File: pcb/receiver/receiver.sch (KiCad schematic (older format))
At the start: 30 parts, among them Q101 Q_PMOS_DSG, U101 TPS63700DRCR, U102 NCP1403SNT1G

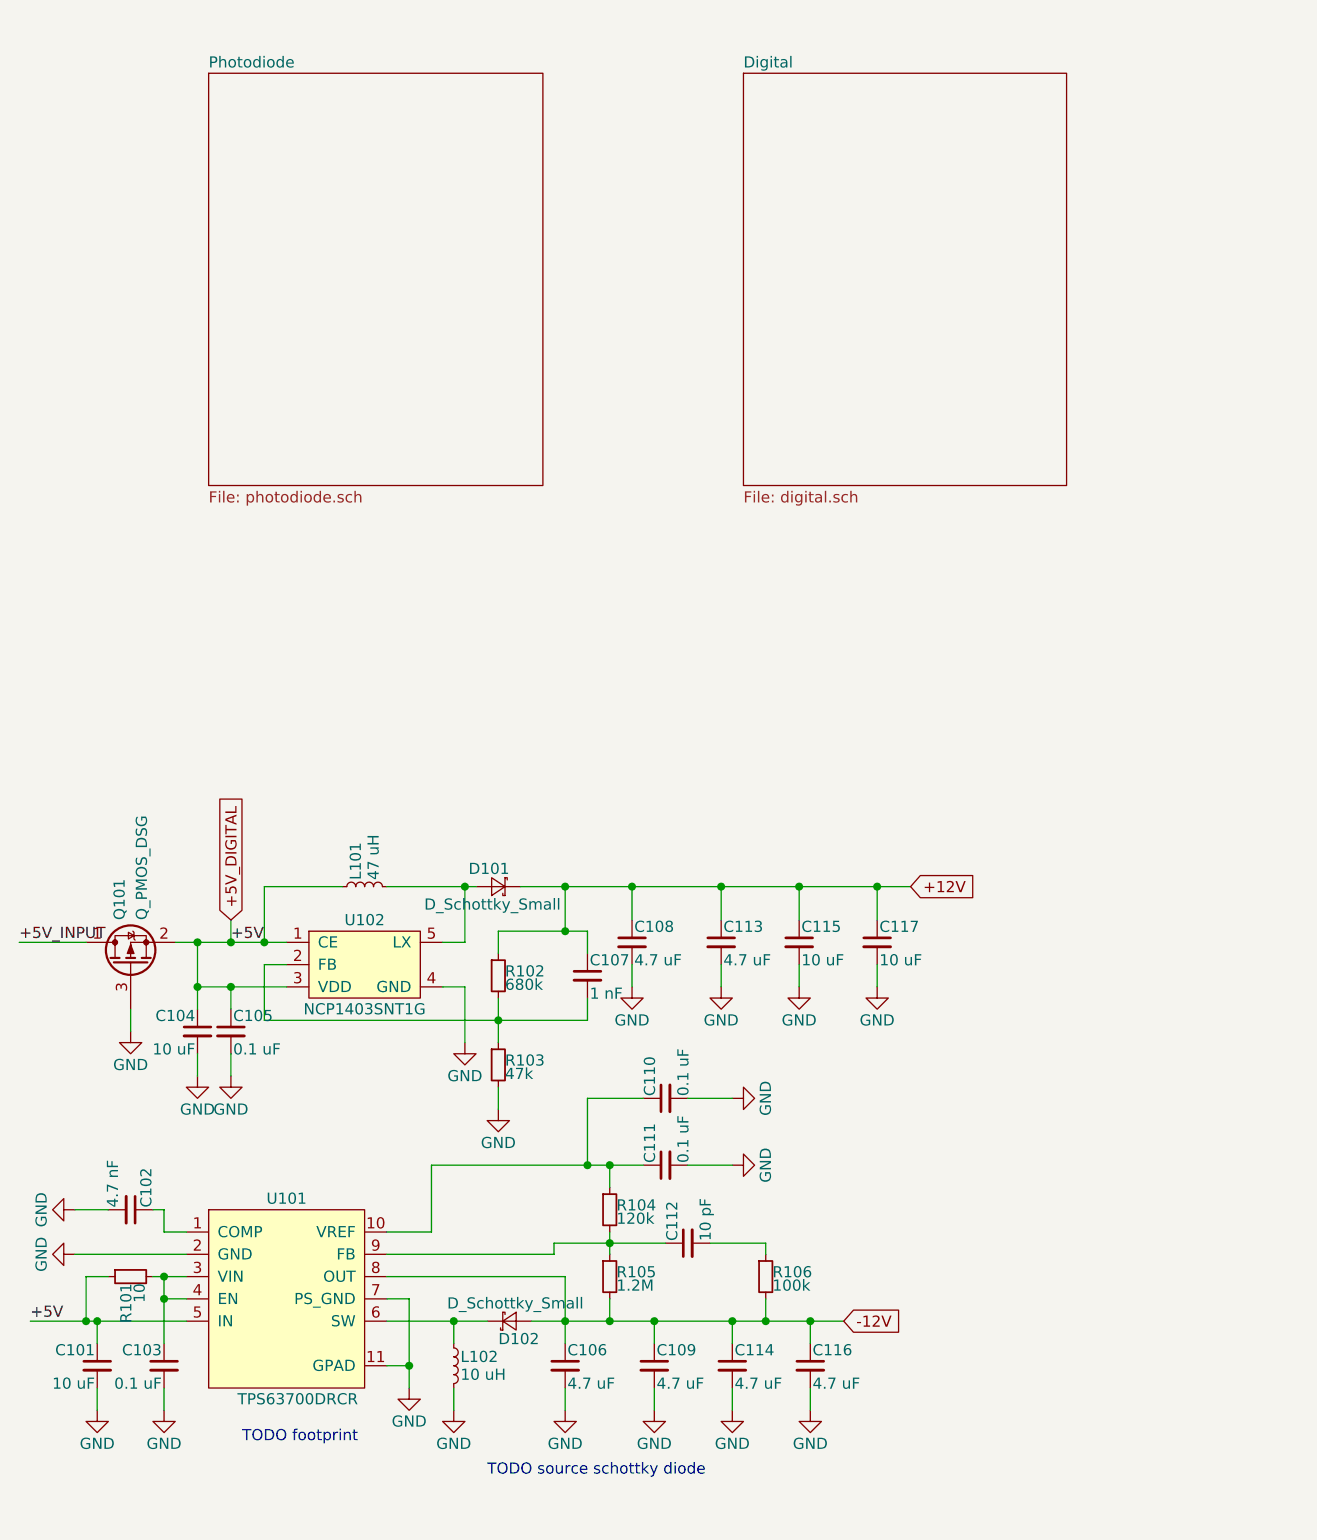
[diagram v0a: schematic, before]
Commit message: Add all components TODO footprint/source everything
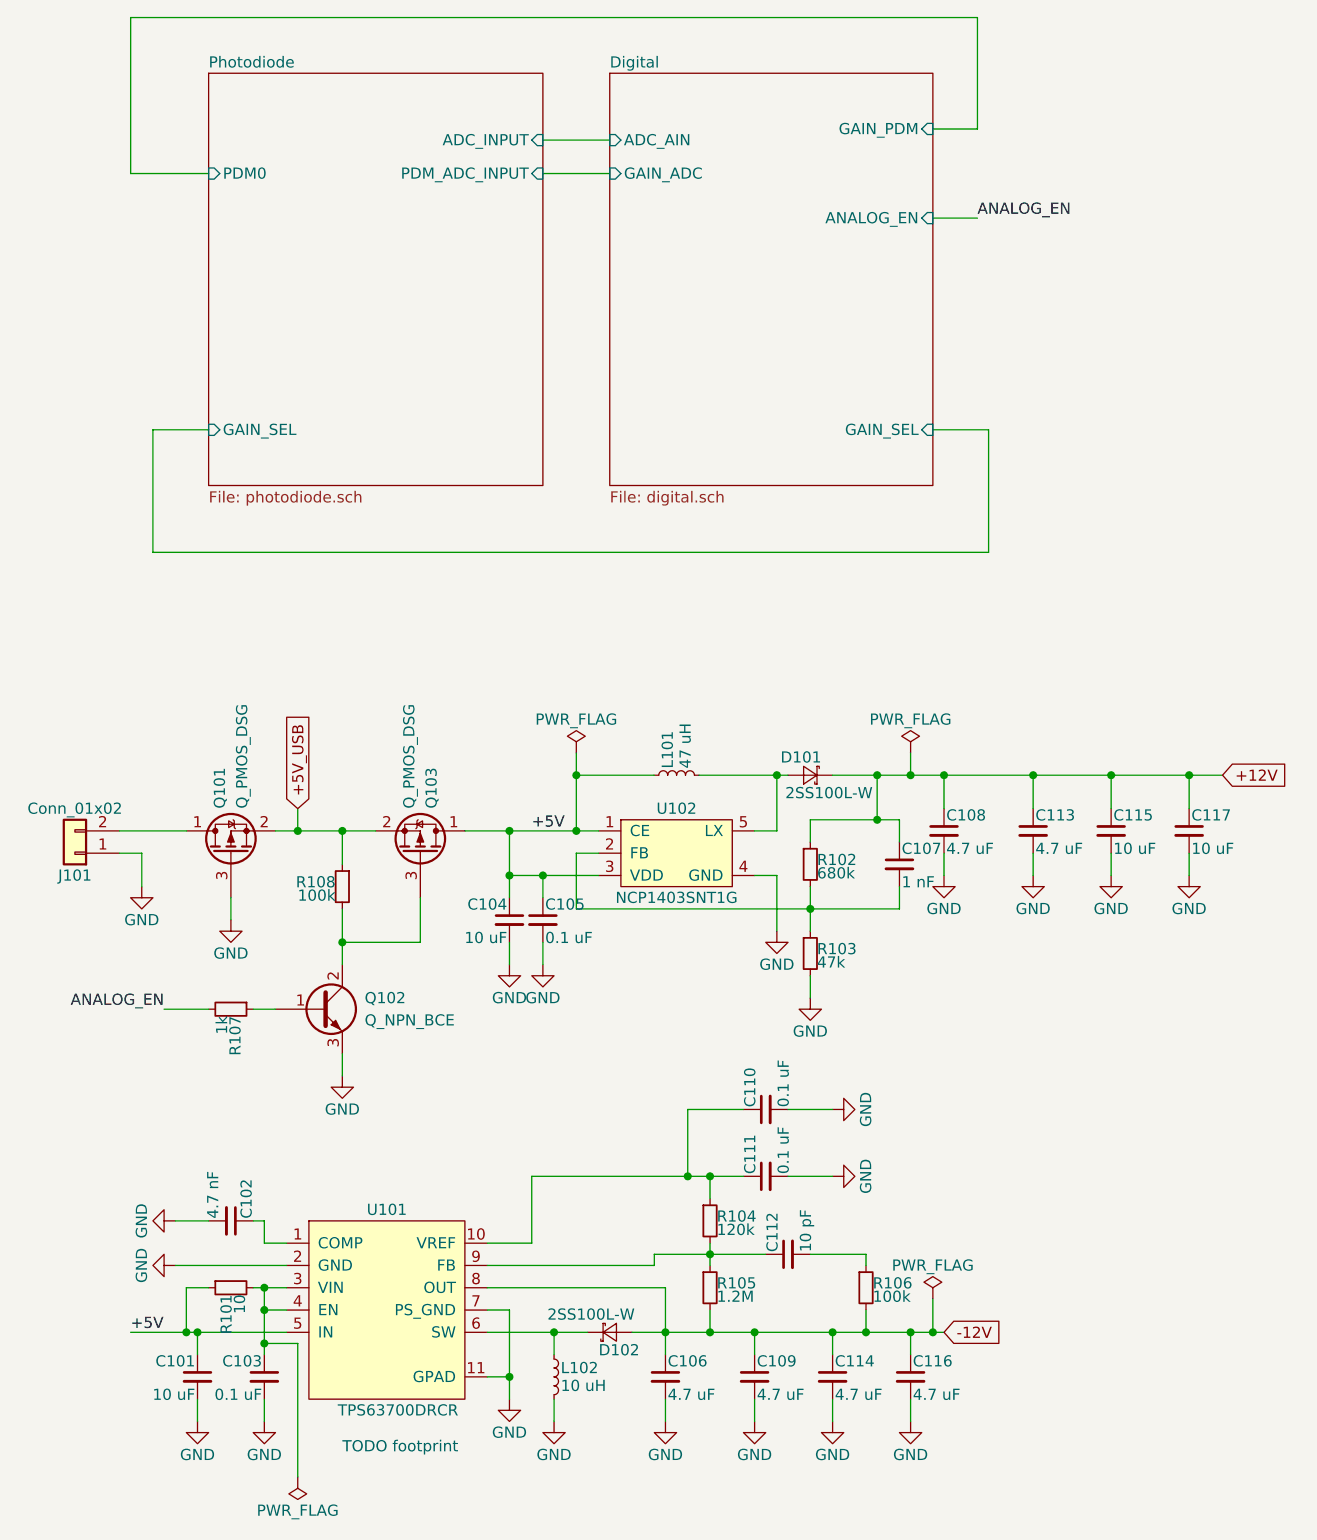
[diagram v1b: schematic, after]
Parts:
- added J101: Conn_01x02, symbol Connector_Generic:Conn_01x02
- added Q102: Q_NPN_BCE, symbol Device:Q_NPN_BCE
- added Q103: Q_PMOS_DSG, symbol Device:Q_PMOS_DSG
- added R107: 1k, symbol Device:R_Small
- added R108: 100k, symbol Device:R_Small
- D101, D102: value D_Schottky_Small -> 2SS100L-W
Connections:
- net GND: now also J101.1 (Pin_1), Q102.3 (E)
- net +5V_DIGITAL renamed +5V
- net +5V: now also Q103.1 (D); no longer Q101.2 (S)
- net +5V_INPUT: no longer names the net of Q101.1 (D)
- net +5V_INPUT: now also J101.2 (Pin_2)
- new net: Q102.2 (C), Q103.3 (G), R108.2
- new net: Q102.1 (B), R107.1
- new net +5V_USB: Q101.2 (S), Q103.2 (S), R108.1
- new net ANALOG_EN: R107.2
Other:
- note removed: "TODO source schottky diode"
- moved on the sheet: C101, C102, C103, C104, C105, C106, C107, C108, C109, C110, C111, C112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
